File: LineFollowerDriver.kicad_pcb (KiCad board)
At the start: 2 copper layers, 18 x 21 mm, 17 parts, among them J1 Conn_01x08_Pin, J2 Conn_01x08_Pin, U1 MT3608, U2 TB6612FNG

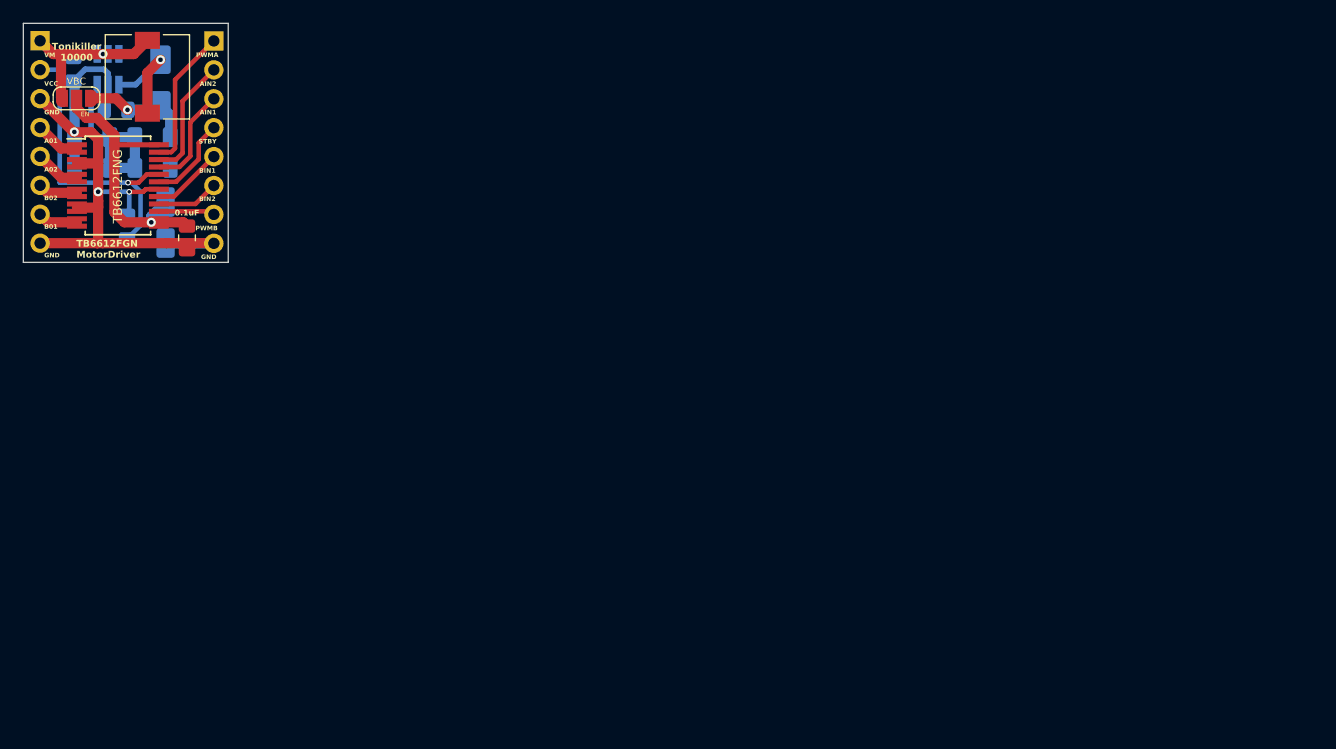
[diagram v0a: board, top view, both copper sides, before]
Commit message: u2
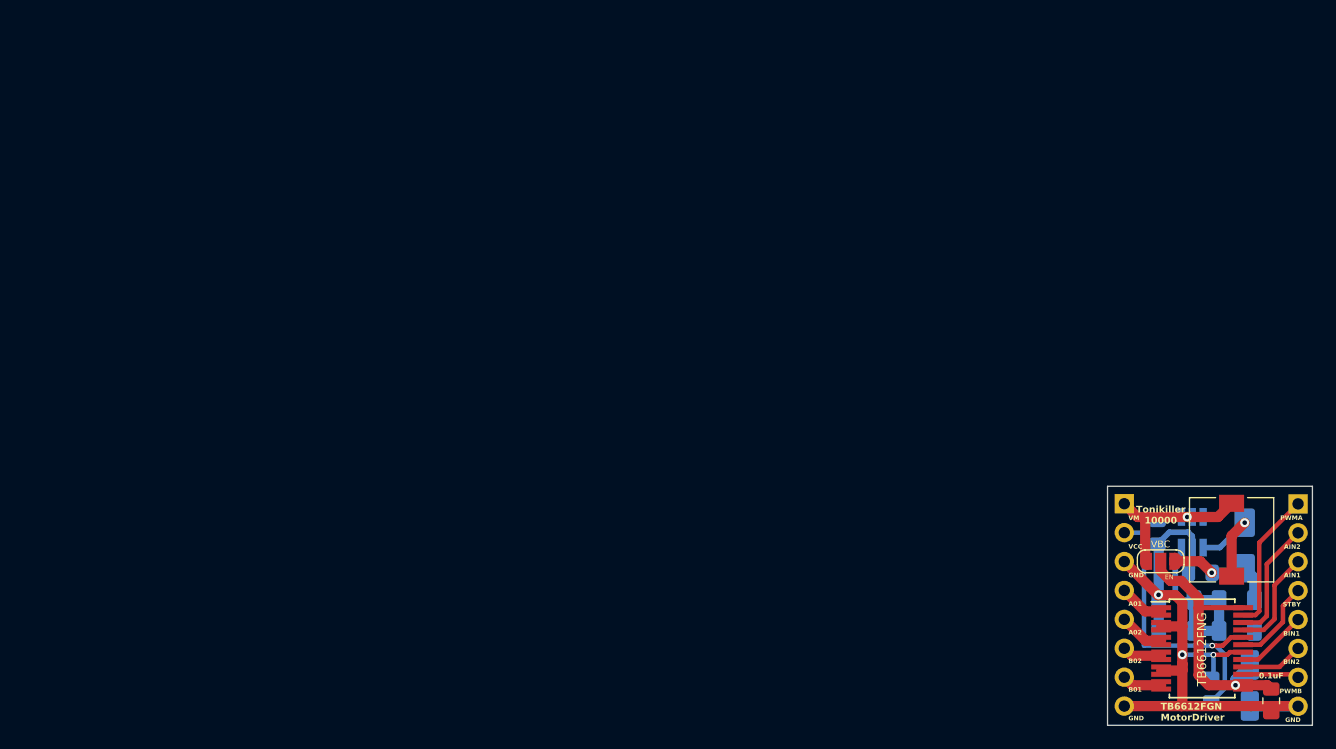
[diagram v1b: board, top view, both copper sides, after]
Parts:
- moved C1 103.6 mm to (145.7, 93.1)
- moved C2 103.6 mm to (149.5, 96.7)
- moved C3 103.6 mm to (153.8, 106.6)
- moved C4 103.6 mm to (150.5, 107.0)
- moved C5 103.6 mm to (155.7, 107.9)
- moved D1 103.6 mm to (153.4, 94.3)
- moved G*** 103.6 mm to (146.9, 106.8)
- moved J2 103.6 mm to (158.1, 90.6)
- moved JP1 103.6 mm to (146.0, 95.7)
- moved L1 103.6 mm to (152.2, 93.8)
- moved R2 103.6 mm to (147.4, 99.1)
- moved R3 103.6 mm to (147.4, 101.8)
- moved U1 103.6 mm to (148.8, 93.1)
- moved U2 103.6 mm to (149.7, 103.3)
- moved J1 103.6 mm to (142.8, 90.6)
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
